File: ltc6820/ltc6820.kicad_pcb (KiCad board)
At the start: 2 copper layers, 40.6 x 19.8 mm, 14 parts, among them J1 Conn_01x06_Pin, J2 Conn_01x02_Pin, T1 78613_3C

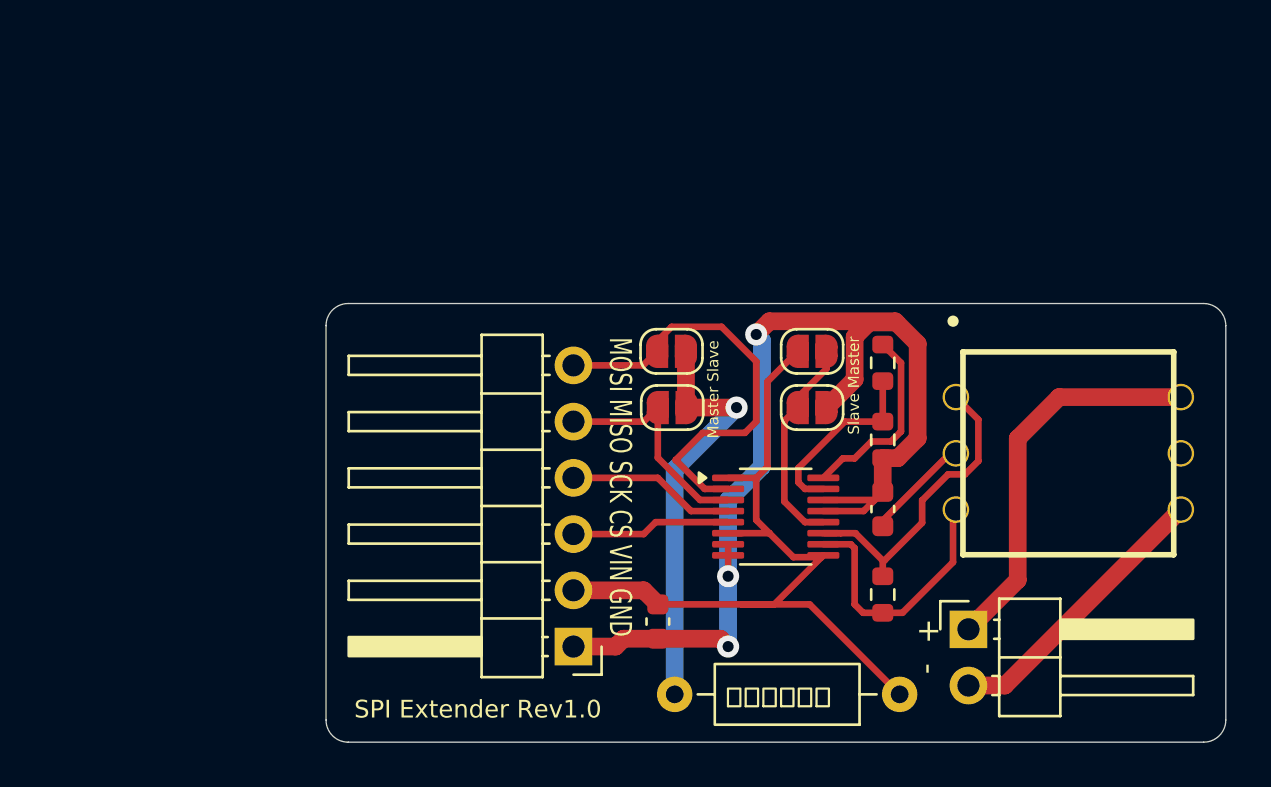
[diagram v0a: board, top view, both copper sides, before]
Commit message: Update: SPI Extender
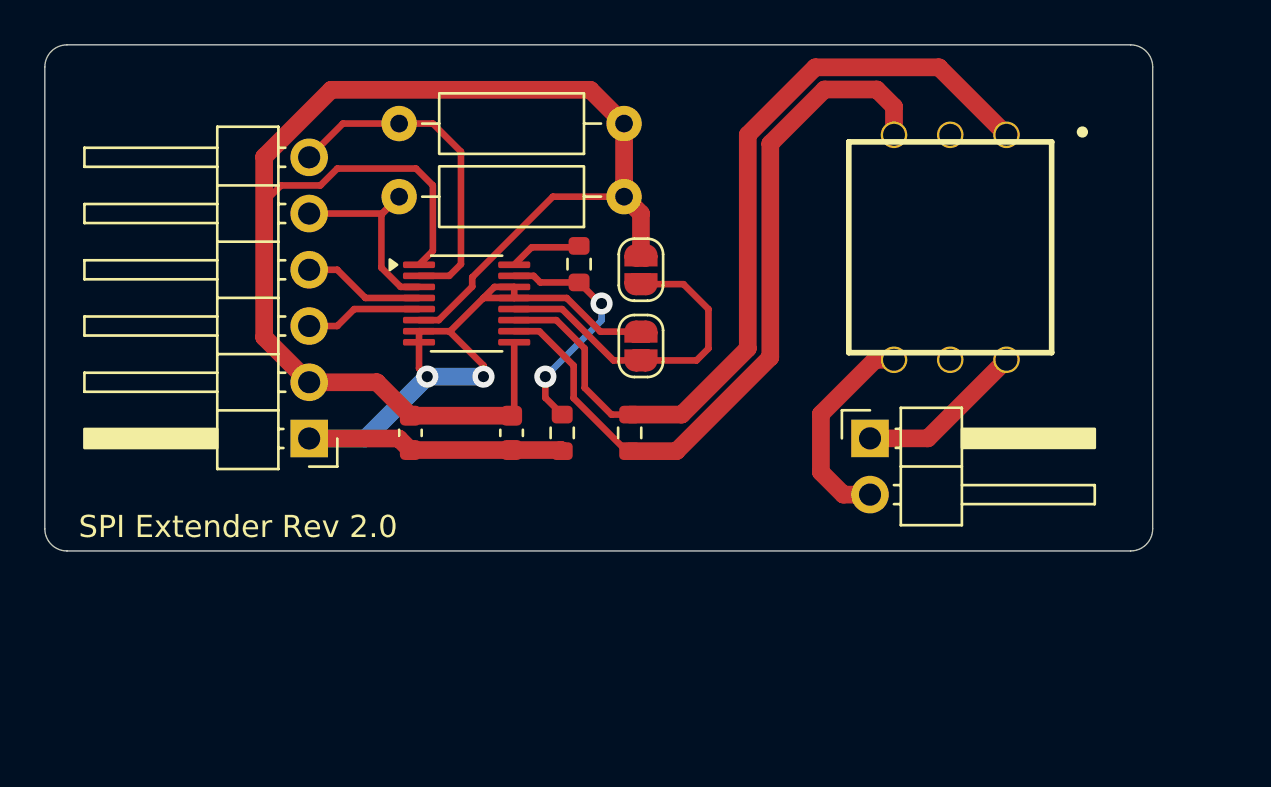
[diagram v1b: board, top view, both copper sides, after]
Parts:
- removed JP1, JP2: SolderJumper_2_Bridged, Jumper:SolderJumper-2_P1.3mm_Open_RoundedPad1.0x1.5mm
- added R5: 10k, Resistor_THT:R_Axial_DIN0207_L6.3mm_D2.5mm_P10.16mm_Horizontal, F.Cu at (78.5, 50.8)
- C1: value 27p -> 0.1u
- R4: value 1k -> 10k
- moved R4 28.6 mm to (78.5, 47.5)
- moved C1 21.6 mm to (68.8, 61.5), turned to -90 degrees
- moved U1 17.0 mm to (71.4, 55.6)
- moved J1 15.2 mm to (64.3, 61.7)
- moved R3 14.5 mm to (75.7, 61.5)
- moved R2 14.4 mm to (76.5, 53.8)
- moved R1 13.6 mm to (78.7, 61.5)
- moved C2 10.8 mm to (73.4, 61.5)
- moved T1 10.7 mm to (93.2, 53.1), turned to -90 degrees
- moved J2 9.70 mm to (89.6, 61.7)
- moved JP3 8.56 mm to (79.2, 54.1), turned to -90 degrees
- moved JP4 8.22 mm to (79.2, 57.5), turned to -90 degrees
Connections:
- C1 pad 1: Net-(C1-Pad1) -> +3V3
- R4 pad 2: Net-(JP1-B) -> MOSI
- T1 pad 2: Net-(C1-Pad1) -> unconnected-(T1-Pad2)
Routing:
- net +3V3: track 36.6 -> 78.9 mm
- net Net-(U1-IP): track 14.0 -> 38.5 mm
- net Net-(U1-IM): track 12.3 -> 34.3 mm
- net Net-(JP1-B): track 18.9 -> 0.00 mm, vias 1 -> 0
- net GND: track 51.0 -> 39.0 mm, vias 3 -> 2
- net IPP: track 17.7 -> 7.63 mm
- net Net-(U1-IBIAS): track 8.65 -> 3.28 mm
- net Net-(C1-Pad1): track 5.23 -> 0.00 mm
- net MSTR: track 10.2 -> 15.2 mm
- net MOSI: track 19.9 -> 15.2 mm
- net IMM: track 12.9 -> 9.58 mm
- net Net-(U1-ICMP): track 8.40 -> 10.8 mm, vias 0 -> 2
- net SCK: track 7.61 -> 5.49 mm
- net CS: track 7.21 -> 5.28 mm
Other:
- board size 40.6 x 19.8 mm -> 50 x 22.9 mm
- board text added: "SPI Extender Rev 2.0"
- board text removed: "+ -"
- board text removed: "MOSI MISO SCK CS VIN GND"
- board text removed: "Master Slave"
- board text removed: "SPI Extender Rev1.0"
- board text removed: "Slave Master"
- board text removed: "ささいな抵抗"
